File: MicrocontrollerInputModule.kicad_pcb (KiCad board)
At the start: 2 copper layers, 31 x 111.4 mm, 369 parts, among them J2 FH34SRJ-12S-0.5SH_50_, SW1 A6H-2101, U1 W25Q16JVUXIQ, U2 RP2040, U3 74AHC125BQ_115, U4 74AHC125BQ_115, Y1 12.000MHz

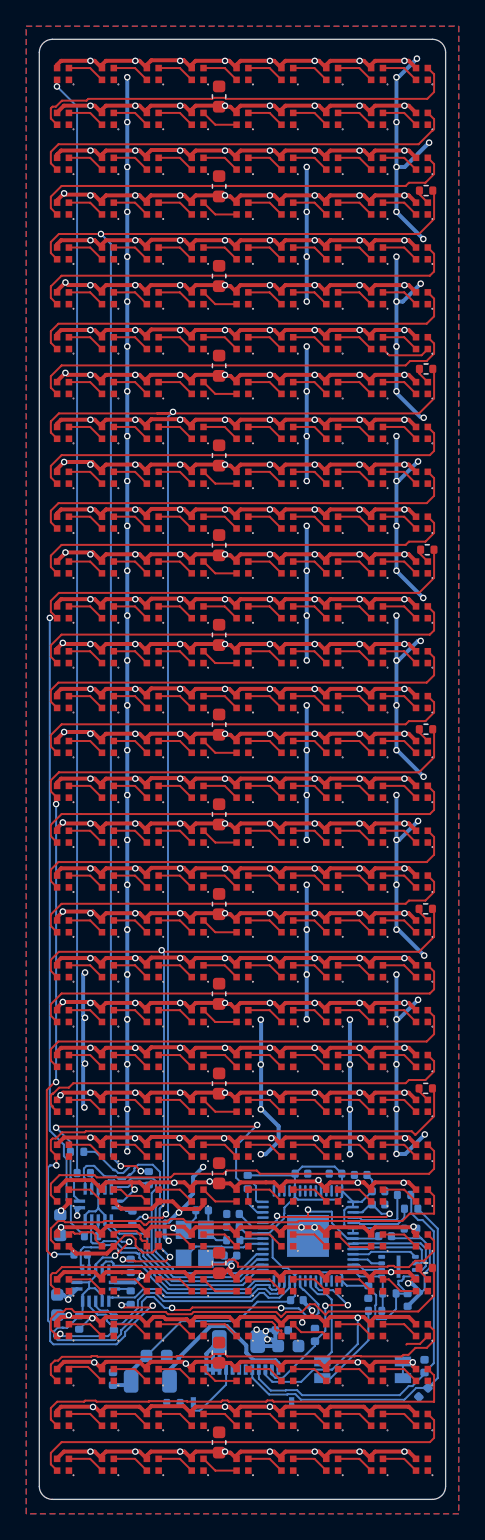
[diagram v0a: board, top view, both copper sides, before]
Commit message: V3 update in preparation for sale
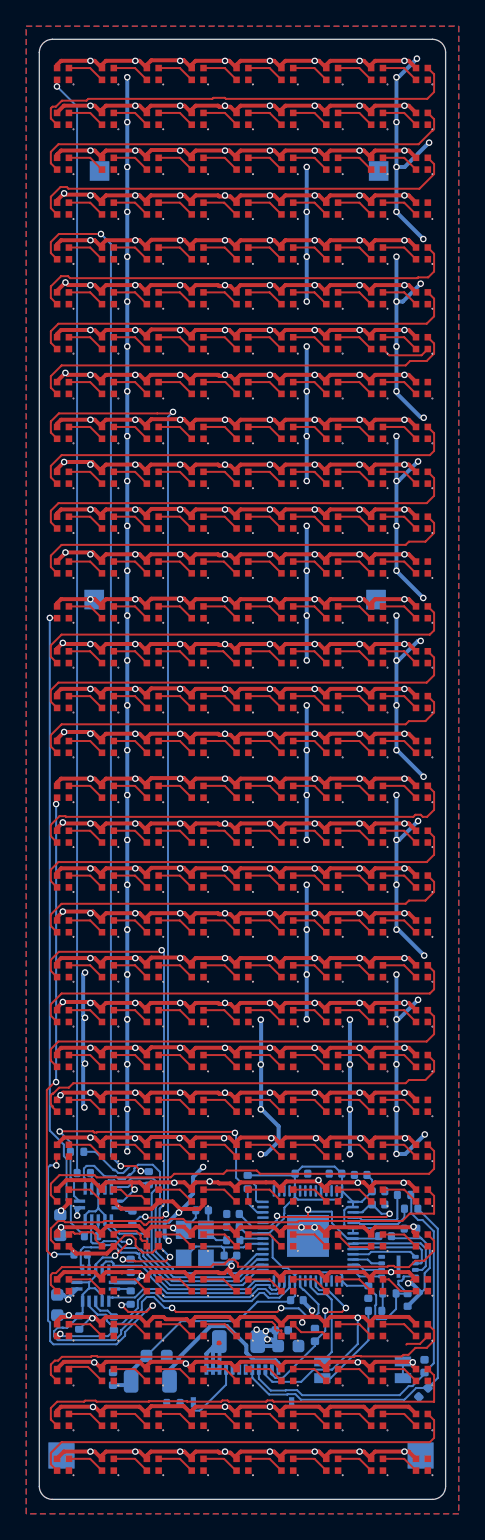
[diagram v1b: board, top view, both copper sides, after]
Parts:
- removed C21, C22, C23, C24, C25, C26, C27, C28, C29, C30, C31, C32, C33, C34, C35, C36: 10uF, Capacitor_SMD:C_0603_1608Metric
- removed R17, R18, R19, R20, R21, R22, R23: 0, Resistor_SMD:R_0402_1005Metric
- added ?: , , F.Cu at (35.2, 28.1)
- added ?: , , F.Cu at (56.5, 28.1)
- added ?: , , F.Cu at (56.3, 60.8)
- added REF**: TestPoint_Pad_2.0x2.0mm, TestPoint:TestPoint_Pad_2.0x2.0mm, B.Cu at (59.7, 126.1)
- added REF**: TestPoint_Pad_1.5x1.5mm, TestPoint:TestPoint_Pad_1.5x1.5mm, B.Cu at (34.8, 60.8)
- added REF**: TestPoint_Pad_2.0x2.0mm, TestPoint:TestPoint_Pad_2.0x2.0mm, B.Cu at (32.3, 126.1)
- N1, N10, N100, N101, N102, N103, N104, N105, N106, N107, N108, N109, N11, N110, N111, N112, N113, N114, N115, N116, N117, N118, N119, N12, N120, N121, N122, N123, N124, N125, N126, N127, N128, N129, N13, N130, N131, N132, N133, N134, N135, N136, N137, N138, N139, N14, N140, N141, N142, N143, N144, N145, N146, N147, N148, N149, N15, N150, N151, N152, N153, N154, N155, N156, N157, N158, N159, N16, N160, N161, N162, N163, N164, N165, N166, N167, N168, N169, N17, N170, N171, N172, N173, N174, N175, N176, N177, N178, N179, N18, N180, N181, N182, N183, N184, N185, N186, N187, N188, N189, N19, N190, N191, N192, N193, N194, N195, N196, N197, N198, N199, N2, N20, N200, N201, N202, N203, N204, N205, N206, N207, N208, N209, N21, N210, N211, N212, N213, N214, N215, N216, N217, N218, N219, N22, N220, N221, N222, N223, N224, N225, N226, N227, N228, N229, N23, N230, N231, N232, N233, N234, N235, N236, N237, N238, N239, N24, N240, N241, N242, N243, N244, N245, N246, N247, N248, N249, N25, N250, N251, N252, N253, N254, N255, N256, N257, N258, N259, N26, N260, N261, N262, N263, N264, N265, N266, N267, N268, N269, N27, N270, N271, N272, N273, N274, N275, N276, N277, N278, N279, N28, N280, N281, N282, N283, N284, N285, N286, N287, N288, N29, N3, N30, N31, N32, N33, N34, N35, N36, N37, N38, N39, N4, N40, N41, N42, N43, N44, N45, N46, N47, N48, N49, N5, N50, N51, N52, N53, N54, N55, N56, N57, N58, N59, N6, N60, N61, N62, N63, N64, N65, N66, N67, N68, N69, N7, N70, N71, N72, N73, N74, N75, N76, N77, N78, N79, N8, N80, N81, N82, N83, N84, N85, N86, N87, N88, N89, N9, N90, N91, N92, N93, N94, N95, N96, N97, N98, N99: value ~ -> SK6805-EC14
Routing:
- net /NeopixelMatrix/STRIP15: track 39.0 -> 4.34 mm
- net /NeopixelMatrix/STRIP9: track 71.0 -> 37.3 mm
- net /NeopixelMatrix/STRIP7: track 82.5 -> 48.8 mm
- net /NeopixelMatrix/STRIP13: track 61.1 -> 27.5 mm
- net /NeopixelMatrix/STRIP3: track 107.5 -> 79.4 mm
- net /NeopixelMatrix/STRIP5: track 99.3 -> 75.5 mm
- net /NeopixelMatrix/STRIP11: track 62.2 -> 38.7 mm
- net /~{OE1}: track 29.9 -> 26.3 mm
- net /NeopixelMatrix/END-STRIP8: track 1.18 -> 0.00 mm
- net /NeopixelMatrix/END-STRIP12: track 1.18 -> 0.00 mm
- net /NeopixelMatrix/END-STRIP2: track 1.18 -> 0.00 mm
- net /NeopixelMatrix/END-STRIP6: track 1.18 -> 0.00 mm
- net /NeopixelMatrix/END-STRIP4: track 1.18 -> 0.00 mm
- net /NeopixelMatrix/END-STRIP14: track 1.18 -> 0.00 mm
- net /NeopixelMatrix/END-STRIP10: track 1.18 -> 0.00 mm
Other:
- board text added: "by Joe Schroedl, v3"
- board text added: "https://jschroedl.com"
- board text removed: "by Joe Schroedl, v2"
- board text removed: "https://github.com/corndog2000"
